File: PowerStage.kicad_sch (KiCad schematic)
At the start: 12 parts, among them J1 Conn_01x01_Pin, J2 Conn_01x01_Pin, J3 Conn_01x01_Pin, J4 Conn_01x01_Pin, J5 Conn_01x01_Pin, Q1 IRF540N

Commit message: new CSV uploaded
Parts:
- Q1: Part Number IRF540N -> IRF540NPBF
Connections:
- new net: L1., L2.
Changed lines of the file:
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@@
 			)
 		)
-		(property "Part Number" "IRF540N"
+		(property "Part Number" "IRF540NPBF"
 			(at 96.52 45.72 0)
 			(effects
@@
 			)
 		)
-		(property "Datasheet" "https://www.microdiode.com/uploadfiles//PDF/SS32-THRU-SS3200-SMA.pdf"
+		(property "Datasheet" "https://services.taiwansemi.com/storage/resources/datasheet/SS32%20SERIES_Q2412.pdf"
 			(at 99.06 57.15 0)
 			(effects

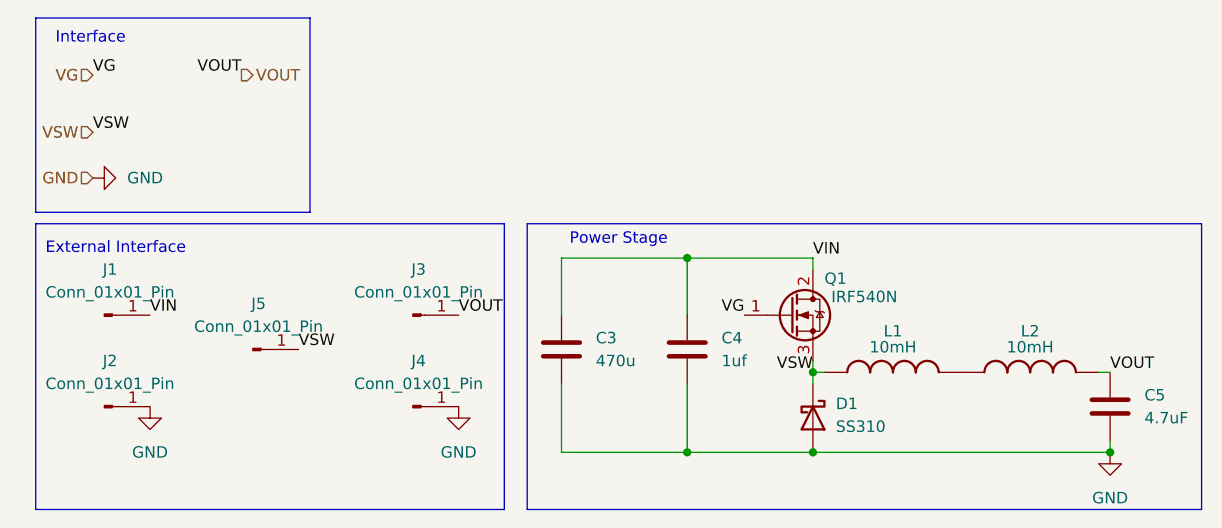
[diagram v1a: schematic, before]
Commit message: Gerber and drill added
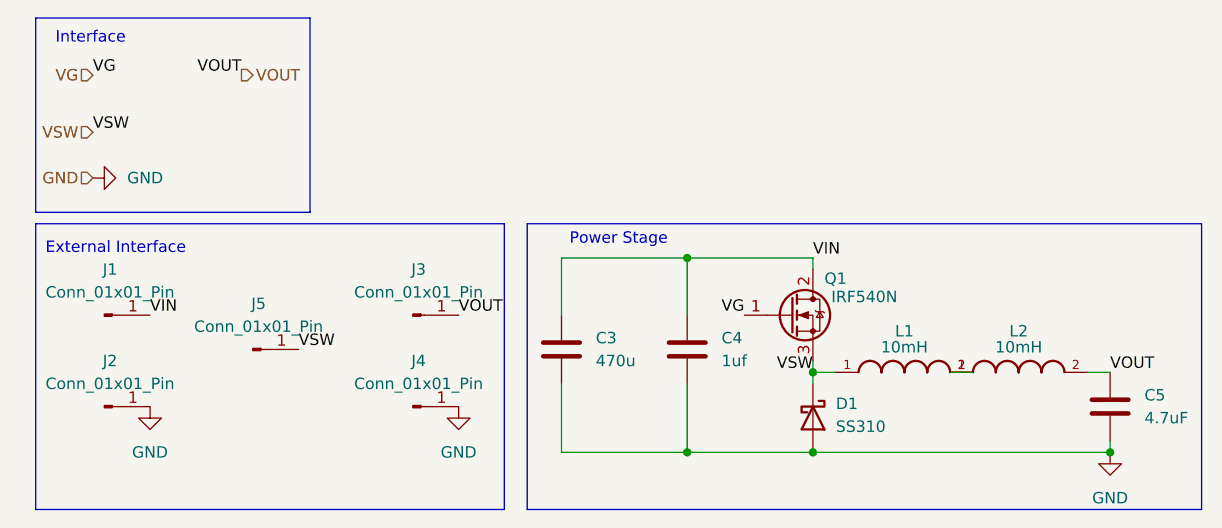
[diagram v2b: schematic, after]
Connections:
- net VOUT: now also L2.2; no longer L2.
- net VSW: now also L1.1; no longer L1.
- new net: L1.2, L2.1
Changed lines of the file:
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@@
 	(wire
 		(pts
-			(xy 130.81 52.07) (xy 132.08 52.07)
+			(xy 129.54 52.07) (xy 132.08 52.07)
 		)
 		(stroke
@@
 	(wire
 		(pts
+			(xy 116.84 52.07) (xy 114.3 52.07)
+		)
+		(stroke
+			(width 0)
+			(type default)
+		)
+	)
+	(wire
+		(pts
 			(xy 85.09 39.37) (xy 99.06 39.37)
 		)
@@
 	(wire
 		(pts
-			(xy 99.06 52.07) (xy 100.33 52.07)
+			(xy 99.06 52.07) (xy 101.6 52.07)
 		)
 		(stroke
@@
 		(lib_name "1140-103K-RC_1")
 		(lib_id "1140-103K-RC:1140-103K-RC")
-		(at 107.95 52.07 90)
+		(at 109.22 52.07 90)
 		(unit 1)
 		(exclude_from_sim no)
@@
 		(dnp no)
 		(property "Reference" "L1"
-			(at 107.95 47.498 90)
+			(at 109.22 47.498 90)
 			(effects
 				(font
@@
 		)
 		(property "Value" "10mH"
-			(at 107.95 49.276 90)
+			(at 109.22 49.276 90)
 			(effects
 				(font
@@
 		)
 		(property "Footprint" "1140-103K-RC:INDRD2921W163D3810H2616P"
-			(at 107.95 52.07 0)
+			(at 109.22 52.07 0)
 			(effects
 				(font
@@
 		)
 		(property "Datasheet" "https://www.bourns.com/docs/Product-Datasheets/1140_series.pdf"
-			(at 107.95 52.07 0)
+			(at 109.22 52.07 0)
 			(effects
 				(font
@@
 		)
 		(property "Description" "FIXED IND 10MH 1A 2.76 OHM TH"
-			(at 107.95 52.07 0)
+			(at 109.22 52.07 0)
 			(effects
 				(font
@@
 		)
 		(property "DigiKey_Part_Number" "M8386-ND"
-			(at 107.95 52.07 0)
+			(at 109.22 52.07 0)
 			(effects
 				(font
@@
 		)
 		(property "SnapEDA_Link" "https://www.snapeda.com/parts/1140-103K-RC/Bourns/view-part/?ref=snap"
-			(at 107.95 52.07 0)
+			(at 109.22 52.07 0)
 			(effects
 				(font
@@
 		)
 		(property "Description_1" "\n                        \n                            CHOKE,RADIAL HIGH CURRENT,10,000 UH, +/-20%, 2.76 OHM DCR MAX | Bourns 1140-103K-RC\n                        \n"
-			(at 107.95 52.07 0)
+			(at 109.22 52.07 0)
 			(effects
 				(font
@@
 		)
 		(property "Package" "Radial Bourns"
-			(at 107.95 52.07 0)
+			(at 109.22 52.07 0)
 			(effects
 				(font
@@
 		)
 		(property "Check_prices" "https://www.snapeda.com/parts/1140-103K-RC/Bourns/view-part/?ref=eda"
-			(at 107.95 52.07 0)
+			(at 109.22 52.07 0)
 			(effects
 				(font
@@
 		)
 		(property "MF" "Bourns"
-			(at 107.95 52.07 0)
+			(at 109.22 52.07 0)
 			(effects
 				(font
@@
 		)
 		(property "MP" "1140-103K-RC"
-			(at 107.95 52.07 0)
+			(at 109.22 52.07 0)
 			(effects
 				(font
@@
 		)
 		(property "MANUFACTURER" "Bourns"
-			(at 107.95 52.07 0)
+			(at 109.22 52.07 0)
 			(effects
 				(font
@@
 		)
 		(property "Part Number" "1140-103K-RC"
-			(at 107.95 52.07 0)
-			(effects
-				(font
-					(size 1.27 1.27)
-				)
-				(hide yes)
-			)
-		)
-		(pin ""
-		)
-		(pin ""
+			(at 109.22 52.07 0)
+			(effects
+				(font
+					(size 1.27 1.27)
+				)
+				(hide yes)
+			)
+		)
+		(pin "1"
+		)
+		(pin "2"
 		)
 		(instances
@@
 	(symbol
 		(lib_id "1140-103K-RC:1140-103K-RC")
-		(at 123.19 52.07 90)
+		(at 121.92 52.07 90)
 		(unit 1)
 		(exclude_from_sim no)
@@
 		(dnp no)
 		(property "Reference" "L2"
-			(at 123.19 47.498 90)
+			(at 121.92 47.498 90)
 			(effects
 				(font
@@
 		)
 		(property "Value" "10mH"
-			(at 123.19 49.276 90)
+			(at 121.92 49.276 90)
 			(effects
 				(font
@@
 		)
 		(property "Footprint" "1140-103K-RC:INDRD2921W163D3810H2616P"
-			(at 123.19 52.07 0)
+			(at 121.92 52.07 0)
 			(effects
 				(font
@@
 		)
 		(property "Datasheet" "https://www.bourns.com/docs/Product-Datasheets/1140_series.pdf"
-			(at 123.19 52.07 0)
+			(at 121.92 52.07 0)
 			(effects
 				(font
@@
 		)
 		(property "Description" "FIXED IND 10MH 1A 2.76 OHM TH"
-			(at 123.19 52.07 0)
+			(at 121.92 52.07 0)
 			(effects
 				(font
@@
 		)
 		(property "DigiKey_Part_Number" "M8386-ND"
-			(at 123.19 52.07 0)
+			(at 121.92 52.07 0)
 			(effects
 				(font
@@
 		)
 		(property "SnapEDA_Link" "https://www.snapeda.com/parts/1140-103K-RC/Bourns/view-part/?ref=snap"
-			(at 123.19 52.07 0)
+			(at 121.92 52.07 0)
 			(effects
 				(font
@@
 		)
 		(property "Description_1" "\n                        \n                            CHOKE,RADIAL HIGH CURRENT,10,000 UH, +/-20%, 2.76 OHM DCR MAX | Bourns 1140-103K-RC\n                        \n"
-			(at 123.19 52.07 0)
+			(at 121.92 52.07 0)
 			(effects
 				(font
@@
 		)
 		(property "Package" "Radial Bourns"
-			(at 123.19 52.07 0)
+			(at 121.92 52.07 0)
 			(effects
 				(font
@@
 		)
 		(property "Check_prices" "https://www.snapeda.com/parts/1140-103K-RC/Bourns/view-part/?ref=eda"
-			(at 123.19 52.07 0)
+			(at 121.92 52.07 0)
 			(effects
 				(font
@@
 		)
 		(property "MF" "Bourns"
-			(at 123.19 52.07 0)
+			(at 121.92 52.07 0)
 			(effects
 				(font
@@
 		)
 		(property "MP" "1140-103K-RC"
-			(at 123.19 52.07 0)
+			(at 121.92 52.07 0)
 			(effects
 				(font
@@
 		)
 		(property "MANUFACTURER" "Bourns"
-			(at 123.19 52.07 0)
+			(at 121.92 52.07 0)
 			(effects
 				(font
@@
 		)
 		(property "Part Number" "1140-103K-RC"
-			(at 123.19 52.07 0)
-			(effects
-				(font
-					(size 1.27 1.27)
-				)
-				(hide yes)
-			)
-		)
-		(pin ""
-		)
-		(pin ""
+			(at 121.92 52.07 0)
+			(effects
+				(font
+					(size 1.27 1.27)
+				)
+				(hide yes)
+			)
+		)
+		(pin "2"
+		)
+		(pin "1"
 		)
 		(instances
